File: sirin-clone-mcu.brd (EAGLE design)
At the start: 101.6 x 55.9 mm, 21 parts

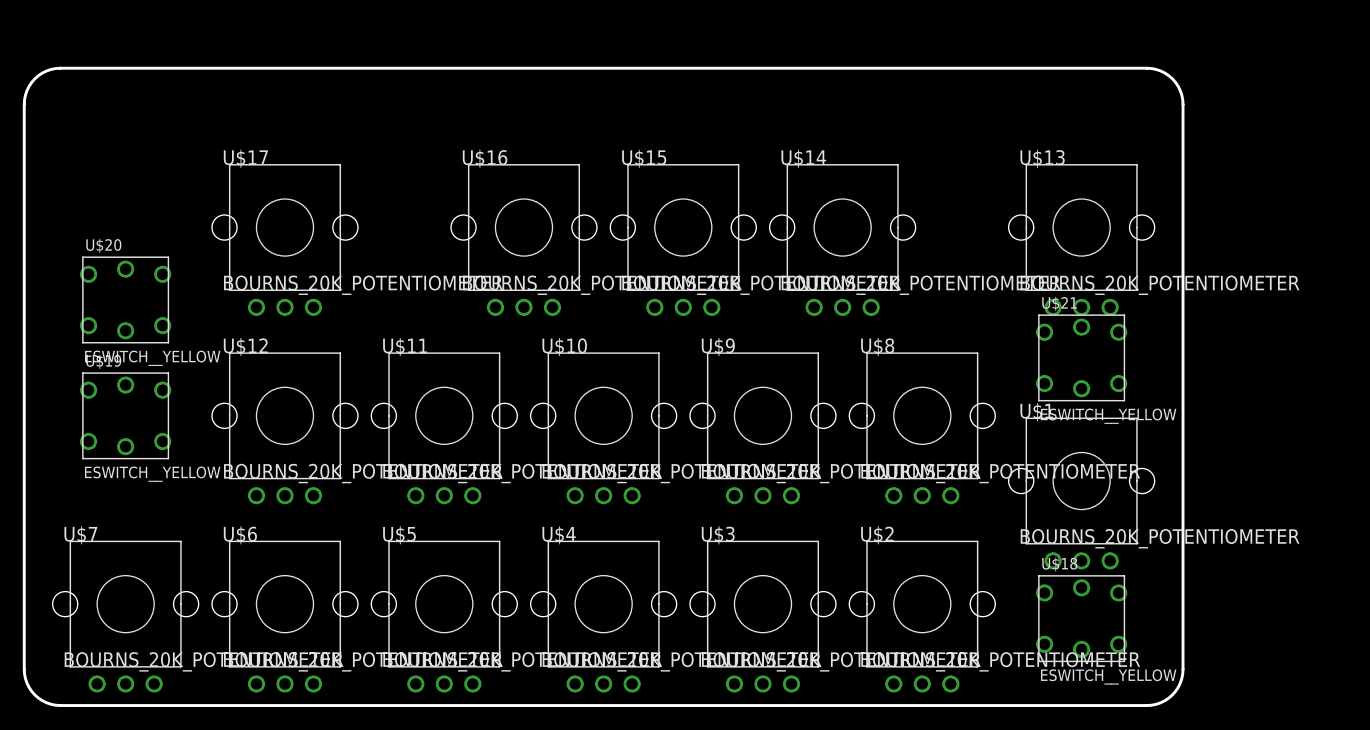
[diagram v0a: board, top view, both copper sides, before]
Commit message: work on lower pcb
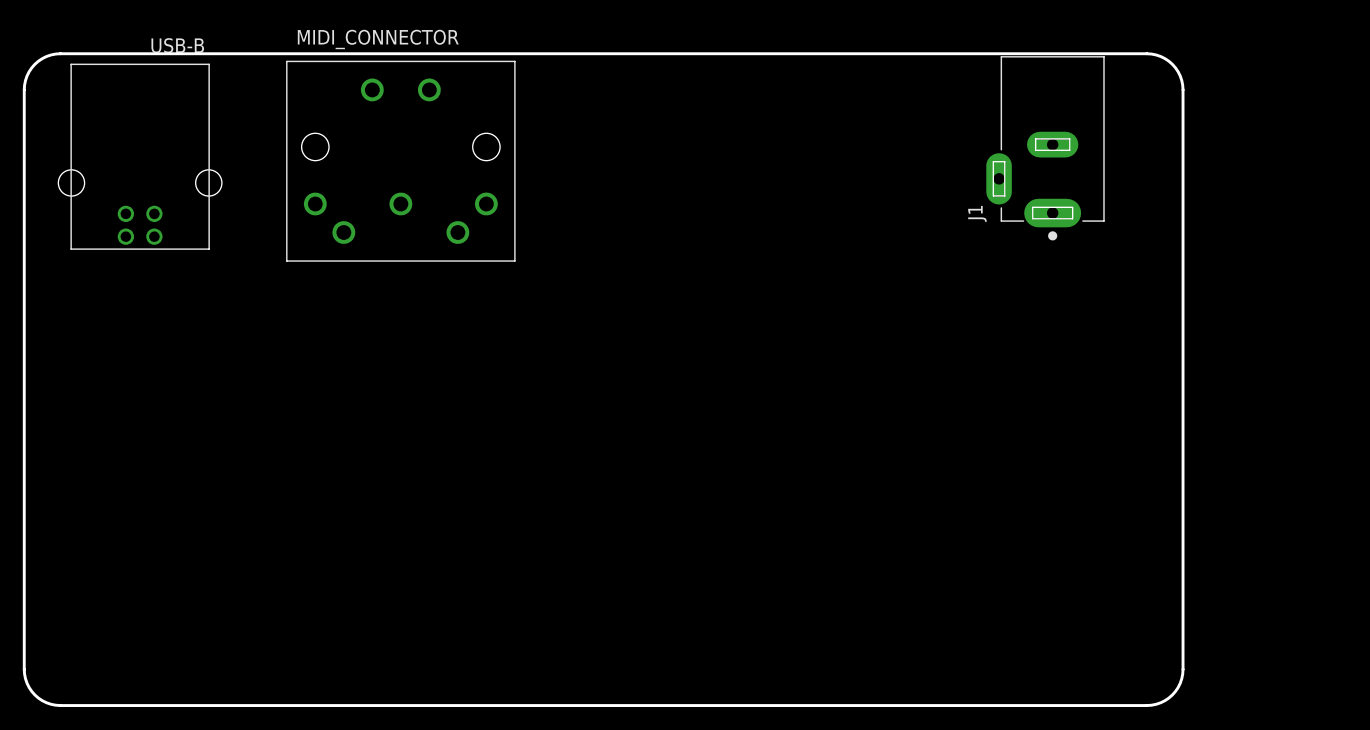
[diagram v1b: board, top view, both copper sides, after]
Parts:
- removed U$10, U$11, U$12, U$13, U$14, U$15, U$16, U$17, U$3, U$4, U$5, U$6, U$7, U$8, U$9: BOURNS_20K_POTENTIOMETER, sirin-clone-library:BOURNS_PTV09
- removed U$18, U$19, U$20, U$21: ESWITCH__YELLOW, sirin-clone-library:ESWITCH_TL1240YQ1JCLR
- added J1: PJ-002A, sirin-clone-library:CUI_PJ-002A
- U$1: value BOURNS_20K_POTENTIOMETER -> MIDI_CONNECTOR; device sirin-clone-library:BOURNS_PTV09 -> sirin-clone-library:DIN_SDS_50J
- U$2: value BOURNS_20K_POTENTIOMETER -> USB-B; device sirin-clone-library:BOURNS_PTV09 -> sirin-clone-library:USB-B
- moved U$2 79.7 mm to (10.2, 49.5), turned to 180 degrees
- moved U$1 68.8 mm to (33.0, 54.0), turned to 180 degrees
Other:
- board size 101.6 x 55.9 mm -> 101.6 x 57.1 mm
